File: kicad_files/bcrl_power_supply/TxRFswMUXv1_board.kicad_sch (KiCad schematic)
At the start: 27 parts, among them J1 OSTVN02A150, J11 5034801600, J2 OSTVN02A150, J3 OSTVN02A150, J4 OSTVN02A150, J5 OSTVN02A150, J6 OSTVN02A150, J7 OSTVN02A150, J8 OSTVN02A150, J9 5034801600, P1 5104338-1, P2 5104338-1, P3 Conn_01x10, P4 Conn_01x10, U1 PDQ10-Q48-S3-D

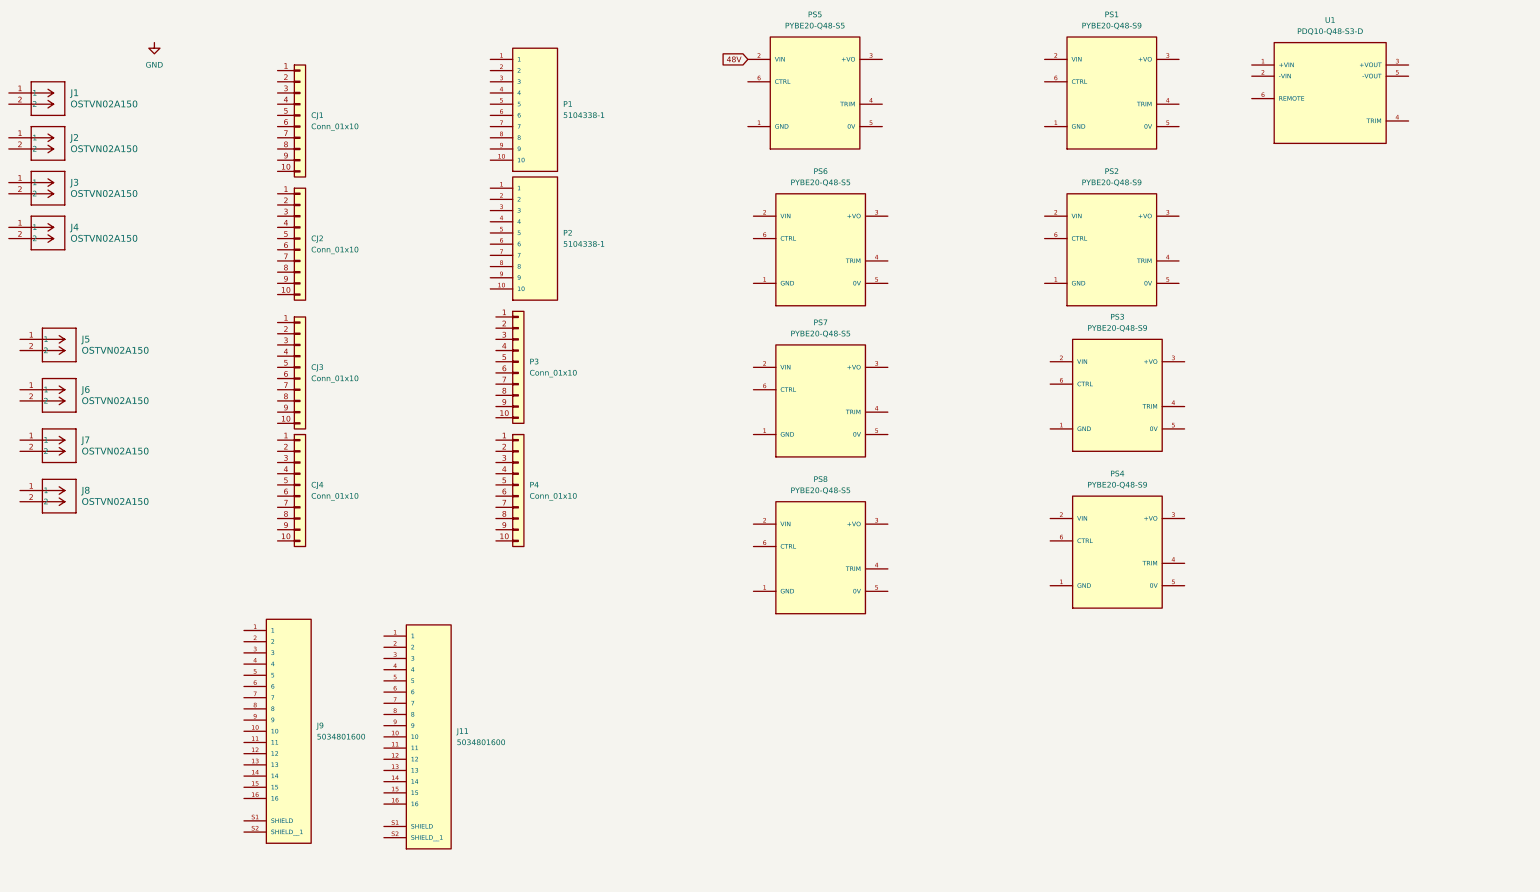
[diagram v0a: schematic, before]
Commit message: fixed path
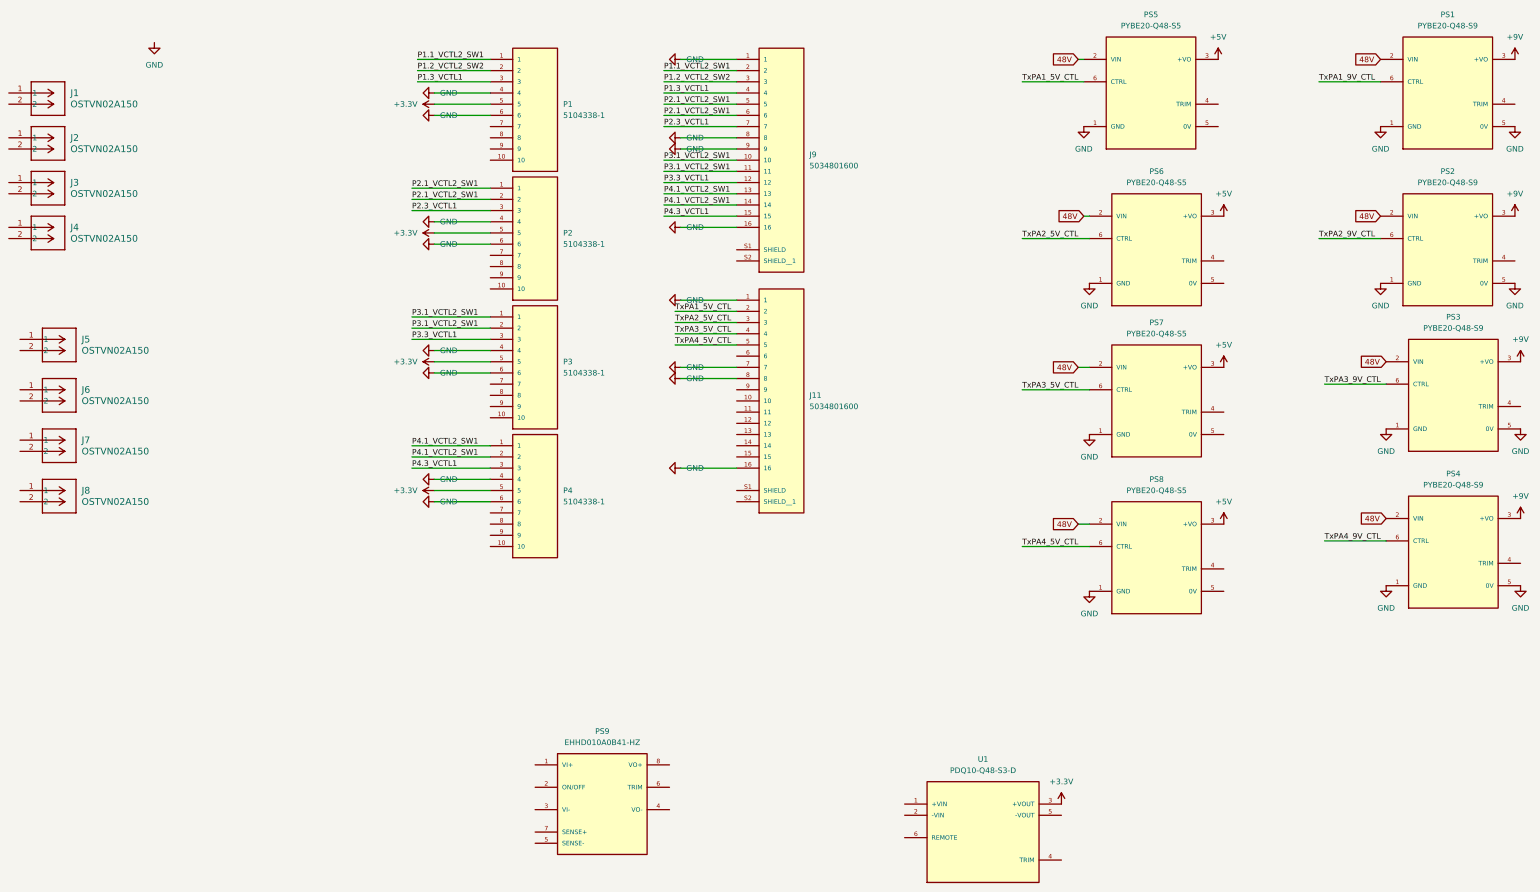
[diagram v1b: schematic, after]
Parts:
- removed CJ1, CJ2, CJ3, CJ4: Conn_01x10, Connector_PinSocket_2.54mm:PinSocket_1x10_P2.54mm_Vertical, symbol Connector_Generic:Conn_01x10
- removed P3, P4: Conn_01x10, Connector_PinSocket_1.27mm:PinSocket_1x10_P1.27mm_Vertical, symbol Connector_Generic:Conn_01x10
- added P3, P4: 5104338-1, symbol BCRL_power_supply:5104338-1
- added PS9: EHHD010A0B41-HZ, symbol BCRL_power_supply:EHHD010A0B41-HZ
- PS1, PS2, PS3, PS4: footprint (none) -> BCRL_power_supply:CONV_PYBE20-Q48-S9
- PS5, PS6, PS7, PS8: footprint PYBE20-Q48-S5:CONV_PYBE20-Q48-S5 -> BCRL_power_supply:CONV_PYBE20-Q48-S5
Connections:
- net 48V: now also PS1.2 (VIN), PS2.2 (VIN), PS3.2 (VIN), PS4.2 (VIN), PS6.2 (VIN), PS7.2 (VIN), PS8.2 (VIN)
- net GND: now also J11.1, J11.16, J11.7, J11.8, J9.1, J9.16, J9.8, J9.9, P1.4, P1.6, P2.4, P2.6, PS1.1 (GND), PS1.5 (0V), PS2.1 (GND), PS2.5 (0V), PS3.1 (GND), PS3.5 (0V), PS4.1 (GND), PS4.5 (0V), PS5.1 (GND), PS6.1 (GND), PS7.1 (GND), PS8.1 (GND), P3.4, P3.6, P4.4, P4.6
- net P3.1_VCTL2_SW1: now reaches J9.10
- net P3.1_VCTL2_SW1: now also J9.11, P3.1, P3.2
- net P3.3_VCTL1: now reaches J9.12
- net P3.3_VCTL1: now also P3.3
- net P4.1_VCTL2_SW1: now reaches J9.13
- net P4.1_VCTL2_SW1: now also J9.14, P4.1, P4.2
- net P4.3_VCTL1: now reaches J9.15
- net P4.3_VCTL1: now also P4.3
- net P1.1_VCTL2_SW1: now reaches J9.2
- net P1.1_VCTL2_SW1: now also P1.1
- net P1.2_VCTL2_SW2: now reaches J9.3
- net P1.2_VCTL2_SW2: now also P1.2
- net P1.3_VCTL1: now reaches J9.4
- net P1.3_VCTL1: now also P1.3
- net P2.1_VCTL2_SW1: now reaches J9.5
- net P2.1_VCTL2_SW1: now also J9.6, P2.1, P2.2
- net P2.3_VCTL1: now reaches J9.7
- net P2.3_VCTL1: now also P2.3
- net +5V: now reaches PS6.3 (+VO)
- net +5V: now also PS5.3 (+VO), PS7.3 (+VO), PS8.3 (+VO)
- net TxPA2_5V_CTL: now reaches PS6.6 (CTRL)
- net TxPA2_5V_CTL: now also J11.3
- net +3.3V: now reaches U1.3 (+VOUT)
- net +3.3V: now also P1.5, P2.5, P3.5, P4.5
- net TxPA4_5V_CTL: now reaches PS8.6 (CTRL)
- net TxPA4_5V_CTL: now also J11.5
- net +9V: now reaches PS2.3 (+VO)
- net +9V: now also PS1.3 (+VO), PS3.3 (+VO), PS4.3 (+VO)
- net TxPA2_9V_CTL: now reaches PS2.6 (CTRL)
- net TxPA1_5V_CTL: now reaches J11.2
- net TxPA1_5V_CTL: now also PS5.6 (CTRL)
- net TxPA3_5V_CTL: now reaches J11.4
- net TxPA3_5V_CTL: now also PS7.6 (CTRL)
- net TxPA3_9V_CTL: now reaches PS3.6 (CTRL)
- net TxPA4_9V_CTL: now reaches PS4.6 (CTRL)
- net TxPA1_9V_CTL: now reaches PS1.6 (CTRL)
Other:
- moved on the sheet: J11, J9, PS1, PS2, PS3, PS4, PS5, PS6, PS7, PS8, U1
